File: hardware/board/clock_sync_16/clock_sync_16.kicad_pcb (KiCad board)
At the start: 4 copper layers, 36 x 28 mm, 47 parts, among them J2 AudioJack3, J3 USB_C_Receptacle_USB2.0, U1 TPD2EUSB30, U2 LP2985-3.3, U3 RP2040, U4 W25Q16JVUXIQ, X1 ECS-TXO-2016

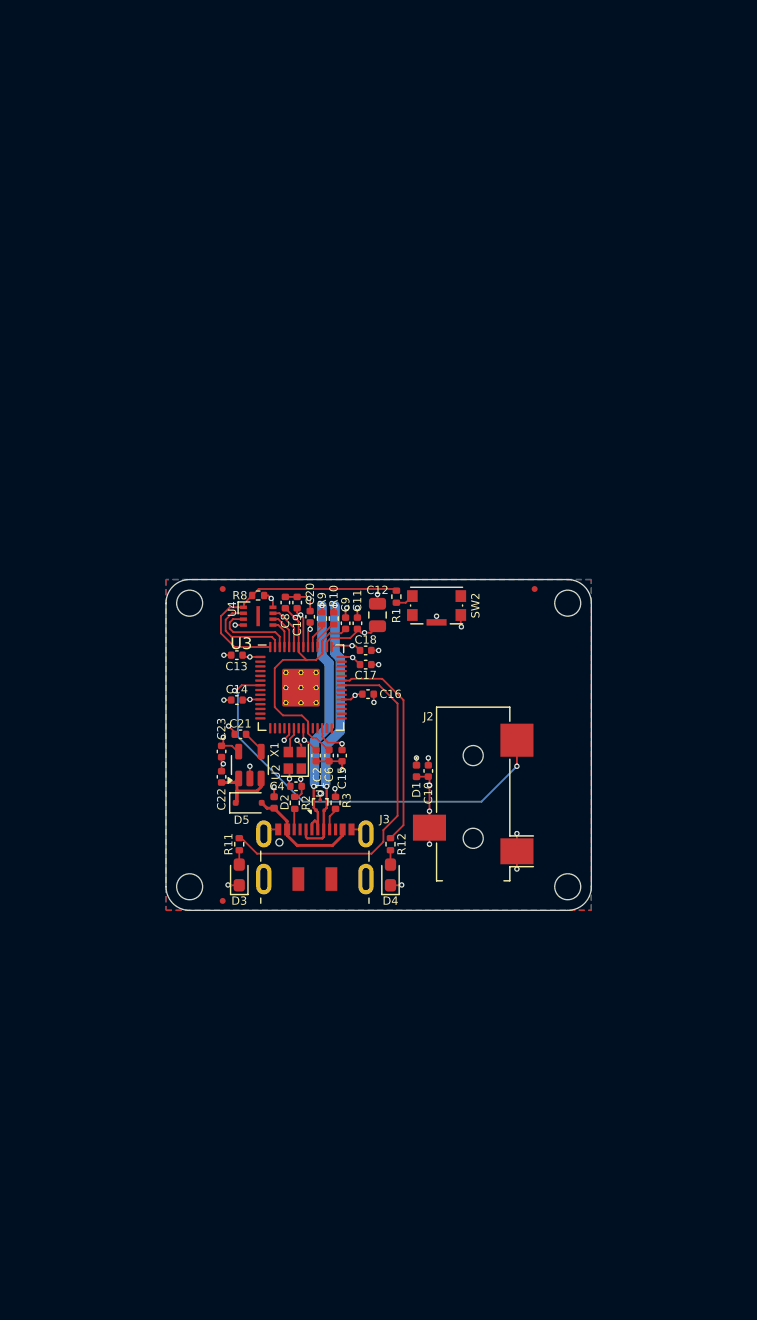
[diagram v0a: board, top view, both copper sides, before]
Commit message: route pcb v0.1
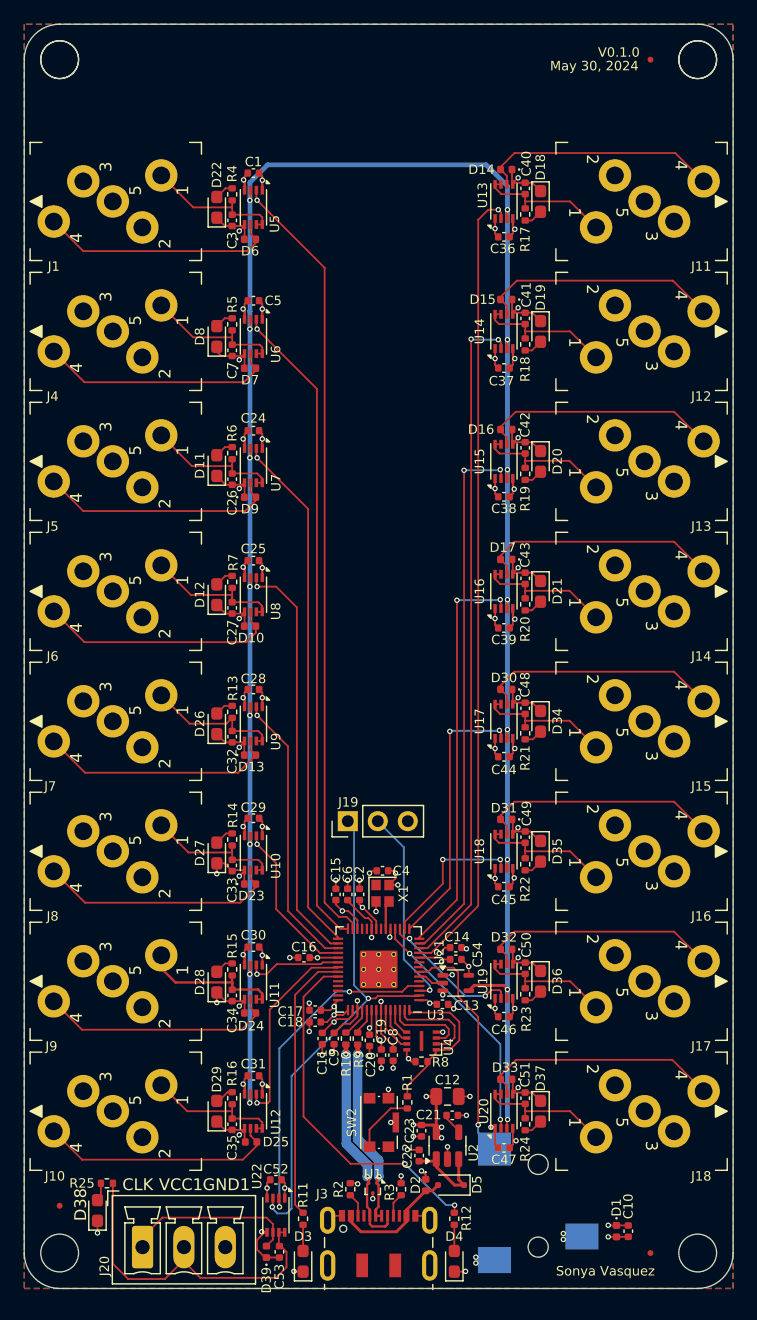
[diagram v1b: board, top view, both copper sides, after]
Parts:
- removed the REF** at (160.0, 84.0)
- removed the REF** at (128.0, 108.0)
- removed the REF** at (160.0, 108.0)
- removed the REF** at (128.0, 84.0)
- added ?: , , F.Cu at (117.0, 38.0)
- added ?: , , F.Cu at (171.0, 38.0)
- added C1: 1uF, Capacitor_SMD:C_0402_1005Metric, F.Cu at (133.4, 47.6)
- added C24: 1uF, Capacitor_SMD:C_0402_1005Metric, F.Cu at (133.4, 69.4)
- added C25: 1uF, Capacitor_SMD:C_0402_1005Metric, F.Cu at (133.4, 80.4)
- added C26: 1uF, Capacitor_SMD:C_0402_1005Metric, F.Cu at (131.6, 73.5)
- added C27: 1uF, Capacitor_SMD:C_0402_1005Metric, F.Cu at (131.6, 84.4)
- added C28: 1uF, Capacitor_SMD:C_0402_1005Metric, F.Cu at (133.4, 91.3)
- added C29: 1uF, Capacitor_SMD:C_0402_1005Metric, F.Cu at (133.4, 102.2)
- added C3: 1uF, Capacitor_SMD:C_0402_1005Metric, F.Cu at (131.6, 51.6)
- added C30: 1uF, Capacitor_SMD:C_0402_1005Metric, F.Cu at (133.4, 113.1)
- added C31: 1uF, Capacitor_SMD:C_0402_1005Metric, F.Cu at (133.4, 124.0)
- added C32: 1uF, Capacitor_SMD:C_0402_1005Metric, F.Cu at (131.6, 95.3)
- added C33: 1uF, Capacitor_SMD:C_0402_1005Metric, F.Cu at (131.6, 106.2)
- added C34: 1uF, Capacitor_SMD:C_0402_1005Metric, F.Cu at (131.6, 117.2)
- added C35: 1uF, Capacitor_SMD:C_0402_1005Metric, F.Cu at (131.6, 128.1)
- added C36: 1uF, Capacitor_SMD:C_0402_1005Metric, F.Cu at (154.6, 53.0)
- added C37: 1uF, Capacitor_SMD:C_0402_1005Metric, F.Cu at (154.6, 64.1)
- added C38: 1uF, Capacitor_SMD:C_0402_1005Metric, F.Cu at (154.6, 75.0)
- added C39: 1uF, Capacitor_SMD:C_0402_1005Metric, F.Cu at (154.6, 86.1)
- added C40: 1uF, Capacitor_SMD:C_0402_1005Metric, F.Cu at (156.4, 48.9)
- added C41: 1uF, Capacitor_SMD:C_0402_1005Metric, F.Cu at (156.4, 59.9)
- added C42: 1uF, Capacitor_SMD:C_0402_1005Metric, F.Cu at (156.4, 70.9)
- added C43: 1uF, Capacitor_SMD:C_0402_1005Metric, F.Cu at (156.4, 81.9)
- added C44: 1uF, Capacitor_SMD:C_0402_1005Metric, F.Cu at (154.6, 97.0)
- added C45: 1uF, Capacitor_SMD:C_0402_1005Metric, F.Cu at (154.6, 108.0)
- added C46: 1uF, Capacitor_SMD:C_0402_1005Metric, F.Cu at (154.6, 119.0)
- added C47: 1uF, Capacitor_SMD:C_0402_1005Metric, F.Cu at (154.6, 130.1)
- added C48: 1uF, Capacitor_SMD:C_0402_1005Metric, F.Cu at (156.4, 92.9)
- added C49: 1uF, Capacitor_SMD:C_0402_1005Metric, F.Cu at (156.4, 103.8)
- added C5: 1uF, Capacitor_SMD:C_0402_1005Metric, F.Cu at (133.4, 58.4)
- added C50: 1uF, Capacitor_SMD:C_0402_1005Metric, F.Cu at (156.4, 114.9)
- added C51: 1uF, Capacitor_SMD:C_0402_1005Metric, F.Cu at (156.4, 125.9)
- added C52: 1uF, Capacitor_SMD:C_0402_1005Metric, F.Cu at (135.3, 132.8)
- added C53: 1uF, Capacitor_SMD:C_0402_1005Metric, F.Cu at (135.6, 138.9)
- added C54: 1uF, Capacitor_SMD:C_0402_1005Metric, F.Cu at (150.5, 114.2)
- added C7: 1uF, Capacitor_SMD:C_0402_1005Metric, F.Cu at (131.6, 62.6)
- added D10: D_TVS, Diode_SMD:D_0402_1005Metric, F.Cu at (133.1, 85.9)
- added D11: LED, LED_SMD:LED_0603_1608Metric_Pad1.05x0.95mm_HandSolder, F.Cu at (130.3, 72.4)
- added D12: LED, LED_SMD:LED_0603_1608Metric_Pad1.05x0.95mm_HandSolder, F.Cu at (130.3, 83.3)
- added D13: D_TVS, Diode_SMD:D_0402_1005Metric, F.Cu at (133.1, 96.9)
- added D14: D_TVS, Diode_SMD:D_0402_1005Metric, F.Cu at (154.8, 47.3)
- added D15: D_TVS, Diode_SMD:D_0402_1005Metric, F.Cu at (154.8, 58.3)
- added D16: D_TVS, Diode_SMD:D_0402_1005Metric, F.Cu at (154.8, 69.3)
- added D17: D_TVS, Diode_SMD:D_0402_1005Metric, F.Cu at (154.8, 80.3)
- added D18: LED, LED_SMD:LED_0603_1608Metric_Pad1.05x0.95mm_HandSolder, F.Cu at (157.7, 50.0)
- added D19: LED, LED_SMD:LED_0603_1608Metric_Pad1.05x0.95mm_HandSolder, F.Cu at (157.7, 61.0)
- added D20: LED, LED_SMD:LED_0603_1608Metric_Pad1.05x0.95mm_HandSolder, F.Cu at (157.7, 72.0)
- added D21: LED, LED_SMD:LED_0603_1608Metric_Pad1.05x0.95mm_HandSolder, F.Cu at (157.7, 83.0)
- added D22: LED, LED_SMD:LED_0603_1608Metric_Pad1.05x0.95mm_HandSolder, F.Cu at (130.3, 50.5)
- added D23: D_TVS, Diode_SMD:D_0402_1005Metric, F.Cu at (133.1, 107.8)
- added D24: D_TVS, Diode_SMD:D_0402_1005Metric, F.Cu at (133.1, 118.7)
- added D25: D_TVS, Diode_SMD:D_0402_1005Metric, F.Cu at (133.2, 129.6)
- added D26: LED, LED_SMD:LED_0603_1608Metric_Pad1.05x0.95mm_HandSolder, F.Cu at (130.3, 94.2)
- added D27: LED, LED_SMD:LED_0603_1608Metric_Pad1.05x0.95mm_HandSolder, F.Cu at (130.3, 105.1)
- added D28: LED, LED_SMD:LED_0603_1608Metric_Pad1.05x0.95mm_HandSolder, F.Cu at (130.3, 116.1)
- added D29: LED, LED_SMD:LED_0603_1608Metric_Pad1.05x0.95mm_HandSolder, F.Cu at (130.3, 127.0)
- added D30: D_TVS, Diode_SMD:D_0402_1005Metric, F.Cu at (154.8, 91.3)
- added D31: D_TVS, Diode_SMD:D_0402_1005Metric, F.Cu at (154.8, 102.3)
- added D32: D_TVS, Diode_SMD:D_0402_1005Metric, F.Cu at (154.8, 113.3)
- added D33: D_TVS, Diode_SMD:D_0402_1005Metric, F.Cu at (154.8, 124.3)
- added D34: LED, LED_SMD:LED_0603_1608Metric_Pad1.05x0.95mm_HandSolder, F.Cu at (157.7, 94.0)
- added D35: LED, LED_SMD:LED_0603_1608Metric_Pad1.05x0.95mm_HandSolder, F.Cu at (157.7, 105.0)
- added D36: LED, LED_SMD:LED_0603_1608Metric_Pad1.05x0.95mm_HandSolder, F.Cu at (157.7, 116.0)
- added D37: LED, LED_SMD:LED_0603_1608Metric_Pad1.05x0.95mm_HandSolder, F.Cu at (157.7, 127.0)
- added D38: LED, LED_SMD:LED_0603_1608Metric_Pad1.05x0.95mm_HandSolder, F.Cu at (120.2, 135.4)
- added D39: D_TVS, Diode_SMD:D_0402_1005Metric, F.Cu at (134.5, 138.9)
- added D6: D_TVS, Diode_SMD:D_0402_1005Metric, F.Cu at (133.1, 53.2)
- added D7: D_TVS, Diode_SMD:D_0402_1005Metric, F.Cu at (133.1, 64.1)
- added D8: LED, LED_SMD:LED_0603_1608Metric_Pad1.05x0.95mm_HandSolder, F.Cu at (130.3, 61.4)
- added D9: D_TVS, Diode_SMD:D_0402_1005Metric, F.Cu at (133.1, 75.0)
- added J1: AudioJack3, kicad_component_library:Jack_3.5mm_Kycon_STX-3680-5NB_Vertical, F.Cu at (121.5, 50.0)
- added J10: AudioJack3, kicad_component_library:Jack_3.5mm_Kycon_STX-3680-5NB_Vertical, F.Cu at (121.5, 127.0)
- added J11: AudioJack3, kicad_component_library:Jack_3.5mm_Kycon_STX-3680-5NB_Vertical, F.Cu at (166.5, 50.0)
- added J12: AudioJack3, kicad_component_library:Jack_3.5mm_Kycon_STX-3680-5NB_Vertical, F.Cu at (166.5, 61.0)
- added J13: AudioJack3, kicad_component_library:Jack_3.5mm_Kycon_STX-3680-5NB_Vertical, F.Cu at (166.5, 72.0)
- added J14: AudioJack3, kicad_component_library:Jack_3.5mm_Kycon_STX-3680-5NB_Vertical, F.Cu at (166.5, 83.0)
- added J15: AudioJack3, kicad_component_library:Jack_3.5mm_Kycon_STX-3680-5NB_Vertical, F.Cu at (166.5, 94.0)
- added J16: AudioJack3, kicad_component_library:Jack_3.5mm_Kycon_STX-3680-5NB_Vertical, F.Cu at (166.5, 105.0)
- added J17: AudioJack3, kicad_component_library:Jack_3.5mm_Kycon_STX-3680-5NB_Vertical, F.Cu at (166.5, 116.0)
- added J18: AudioJack3, kicad_component_library:Jack_3.5mm_Kycon_STX-3680-5NB_Vertical, F.Cu at (166.5, 127.0)
- added J19: Conn_01x03_Male, Connector_PinHeader_2.54mm:PinHeader_1x03_P2.54mm_Vertical, F.Cu at (141.4, 102.5)
- added J20: Conn_01x03_Female, Connector_Phoenix_MC:PhoenixContact_MCV_1,5_3-G-3.5_1x03_P3.50mm_Vertical, F.Cu at (124.0, 138.5)
- added J4: AudioJack3, kicad_component_library:Jack_3.5mm_Kycon_STX-3680-5NB_Vertical, F.Cu at (121.5, 61.0)
- added J5: AudioJack3, kicad_component_library:Jack_3.5mm_Kycon_STX-3680-5NB_Vertical, F.Cu at (121.5, 72.0)
- added J6: AudioJack3, kicad_component_library:Jack_3.5mm_Kycon_STX-3680-5NB_Vertical, F.Cu at (121.5, 83.0)
- added J7: AudioJack3, kicad_component_library:Jack_3.5mm_Kycon_STX-3680-5NB_Vertical, F.Cu at (121.5, 94.0)
- added J8: AudioJack3, kicad_component_library:Jack_3.5mm_Kycon_STX-3680-5NB_Vertical, F.Cu at (121.5, 105.0)
- added J9: AudioJack3, kicad_component_library:Jack_3.5mm_Kycon_STX-3680-5NB_Vertical, F.Cu at (121.5, 116.0)
- added R13: R, Resistor_SMD:R_0402_1005Metric, F.Cu at (131.6, 93.2)
- added R14: R, Resistor_SMD:R_0402_1005Metric, F.Cu at (131.6, 104.0)
- added R15: R, Resistor_SMD:R_0402_1005Metric, F.Cu at (131.6, 115.0)
- added R16: R, Resistor_SMD:R_0402_1005Metric, F.Cu at (131.6, 125.9)
- added R17: R, Resistor_SMD:R_0402_1005Metric, F.Cu at (156.4, 51.1)
- added R18: R, Resistor_SMD:R_0402_1005Metric, F.Cu at (156.4, 62.1)
- added R19: R, Resistor_SMD:R_0402_1005Metric, F.Cu at (156.4, 73.1)
- added R20: R, Resistor_SMD:R_0402_1005Metric, F.Cu at (156.4, 84.1)
- added R21: R, Resistor_SMD:R_0402_1005Metric, F.Cu at (156.4, 95.0)
- added R22: R, Resistor_SMD:R_0402_1005Metric, F.Cu at (156.4, 106.1)
- added R23: R, Resistor_SMD:R_0402_1005Metric, F.Cu at (156.4, 117.1)
- added R24: R, Resistor_SMD:R_0402_1005Metric, F.Cu at (156.4, 128.1)
- added R25: R, Resistor_SMD:R_0402_1005Metric, F.Cu at (121.0, 133.1)
- added R4: R, Resistor_SMD:R_0402_1005Metric, F.Cu at (131.6, 49.4)
- added R5: R, Resistor_SMD:R_0402_1005Metric, F.Cu at (131.6, 60.4)
- added R6: R, Resistor_SMD:R_0402_1005Metric, F.Cu at (131.6, 71.3)
- added R7: R, Resistor_SMD:R_0402_1005Metric, F.Cu at (131.6, 82.2)
- added REF**: MountingHole_3.2mm_M3_DIN965, MountingHole:MountingHole_3.2mm_M3_DIN965, F.Cu at (117.0, 38.0)
- added REF**: MountingHole_3.2mm_M3_DIN965, MountingHole:MountingHole_3.2mm_M3_DIN965, F.Cu at (117.0, 139.0)
- added REF**: MountingHole_3.2mm_M3_DIN965, MountingHole:MountingHole_3.2mm_M3_DIN965, F.Cu at (171.0, 38.0)
- added REF**: MountingHole_3.2mm_M3_DIN965, MountingHole:MountingHole_3.2mm_M3_DIN965, F.Cu at (171.0, 139.0)
- added U10: ISO6521FREUR, kicad_component_library:DFN-8_3x2mm_P0.5mm, F.Cu at (133.4, 105.1)
- added U11: ISO6521FREUR, kicad_component_library:DFN-8_3x2mm_P0.5mm, F.Cu at (133.4, 116.1)
- added U12: ISO6521FREUR, kicad_component_library:DFN-8_3x2mm_P0.5mm, F.Cu at (133.4, 127.0)
- added U13: ISO6521FREUR, kicad_component_library:DFN-8_3x2mm_P0.5mm, F.Cu at (154.6, 50.0)
- added U14: ISO6521FREUR, kicad_component_library:DFN-8_3x2mm_P0.5mm, F.Cu at (154.6, 61.0)
- added U15: ISO6521FREUR, kicad_component_library:DFN-8_3x2mm_P0.5mm, F.Cu at (154.6, 72.0)
- added U16: ISO6521FREUR, kicad_component_library:DFN-8_3x2mm_P0.5mm, F.Cu at (154.6, 83.0)
- added U17: ISO6521FREUR, kicad_component_library:DFN-8_3x2mm_P0.5mm, F.Cu at (154.6, 94.0)
- added U18: ISO6521FREUR, kicad_component_library:DFN-8_3x2mm_P0.5mm, F.Cu at (154.6, 105.0)
- added U19: ISO6521FREUR, kicad_component_library:DFN-8_3x2mm_P0.5mm, F.Cu at (154.6, 116.0)
- added U20: ISO6521FREUR, kicad_component_library:DFN-8_3x2mm_P0.5mm, F.Cu at (154.6, 127.0)
- added U21: SN74LVC1G125DCK, Package_TO_SOT_SMD:Texas_R-PDSO-G5_DCK-5, F.Cu at (150.5, 116.2)
- added U22: ISO6521FREUR, kicad_component_library:DFN-8_3x2mm_P0.5mm, F.Cu at (135.3, 135.8)
- added U5: ISO6521FREUR, kicad_component_library:DFN-8_3x2mm_P0.5mm, F.Cu at (133.4, 50.5)
- added U6: ISO6521FREUR, kicad_component_library:DFN-8_3x2mm_P0.5mm, F.Cu at (133.4, 61.4)
- added U7: ISO6521FREUR, kicad_component_library:DFN-8_3x2mm_P0.5mm, F.Cu at (133.4, 72.4)
- added U8: ISO6521FREUR, kicad_component_library:DFN-8_3x2mm_P0.5mm, F.Cu at (133.4, 83.3)
- added U9: ISO6521FREUR, kicad_component_library:DFN-8_3x2mm_P0.5mm, F.Cu at (133.4, 94.2)
- J2: moved to B.Cu
- moved FID3 79.9 mm to (167.0, 38.0)
- moved FID2 57.0 mm to (167.0, 139.0)
- moved FID1 54.0 mm to (117.0, 135.0)
- moved SW2 44.0 mm to (144.0, 128.0), turned to -90 degrees
- moved R1 42.8 mm to (146.4, 126.2)
- moved C10 42.5 mm to (165.1, 137.2)
- moved D1 42.5 mm to (164.1, 137.2)
- moved R8 41.8 mm to (147.6, 122.8), turned to 180 degrees
- moved C12 41.2 mm to (149.8, 125.8), turned to 0 degrees
- moved C8 39.4 mm to (145.2, 122.2), turned to 90 degrees
- moved C19 39.0 mm to (144.2, 122.2), turned to 90 degrees
- moved U4 38.5 mm to (147.6, 121.0), turned to 180 degrees
- moved C21 36.9 mm to (150.2, 127.3), turned to 0 degrees
- moved D5 36.6 mm to (150.1, 133.2), turned to 180 degrees
- moved U2 36.3 mm to (149.8, 129.9)
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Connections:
- net +3V3 renamed +3.3V
- net /Harp Core RP2040 + USB/HARP_CLK_SYNC renamed /Harp Core RP2040 + USB/HARP_CLKIN_SYNC
- U3 pad 11: unconnected-(U3-GPIO8-Pad11) -> /Clock Outputs 8 - 16/CH8_CONNECTED
- U3 pad 12: unconnected-(U3-GPIO9-Pad12) -> /Clock Outputs 8 - 16/CH9_CONNECTED
- U3 pad 13: unconnected-(U3-GPIO10-Pad13) -> /Clock Outputs 8 - 16/CH10_CONNECTED
- U3 pad 14: unconnected-(U3-GPIO11-Pad14) -> /Clock Outputs 8 - 16/CH11_CONNECTED
- U3 pad 15: unconnected-(U3-GPIO12-Pad15) -> /Clock Outputs 8 - 16/CH12_CONNECTED
- U3 pad 16: unconnected-(U3-GPIO13-Pad16) -> /Clock Outputs 8 - 16/CH13_CONNECTED
- U3 pad 17: unconnected-(U3-GPIO14-Pad17) -> /Clock Outputs 8 - 16/CH14_CONNECTED
- U3 pad 18: unconnected-(U3-GPIO15-Pad18) -> /Clock Outputs 8 - 16/CH15_CONNECTED
- U3 pad 2: unconnected-(U3-GPIO0-Pad2) -> /Harp Core RP2040 + USB/SLOW_CLKOUT
- U3 pad 27: unconnected-(U3-GPIO16-Pad27) -> /Clock Outputs 0 - 7/CH0_CONNECTED
- U3 pad 28: unconnected-(U3-GPIO17-Pad28) -> /Clock Outputs 0 - 7/CH1_CONNECTED
- U3 pad 29: unconnected-(U3-GPIO18-Pad29) -> /Clock Outputs 0 - 7/CH2_CONNECTED
- U3 pad 3: unconnected-(U3-GPIO1-Pad3) -> /Harp Core RP2040 + USB/UART0_RXD
- U3 pad 30: unconnected-(U3-GPIO19-Pad30) -> /Clock Outputs 0 - 7/CH3_CONNECTED
- U3 pad 31: unconnected-(U3-GPIO20-Pad31) -> /Clock Outputs 0 - 7/CH4_CONNECTED
- U3 pad 32: unconnected-(U3-GPIO21-Pad32) -> /Clock Outputs 0 - 7/CH5_CONNECTED
- U3 pad 34: unconnected-(U3-GPIO22-Pad34) -> /Clock Outputs 0 - 7/CH6_CONNECTED
- U3 pad 35: unconnected-(U3-GPIO23-Pad35) -> /Clock Outputs 0 - 7/CH7_CONNECTED
- U3 pad 4: unconnected-(U3-GPIO2-Pad4) -> /Harp Core RP2040 + USB/SLOW_CLKOUT_CONNECTED
- U3 pad 6: unconnected-(U3-GPIO4-Pad6) -> /Harp Core RP2040 + USB/HARP_CLKOUT
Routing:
- net HARP_CLKOUT: track 0.00 -> 196.3 mm, vias 0 -> 16
- net /Clock Outputs 8 - 16/CH8_CONNECTED: track 0.00 -> 67.6 mm, vias 0 -> 1
- net /Clock Outputs 0 - 7/CH0_CONNECTED: track 0.00 -> 66.3 mm, vias 0 -> 1
- net /Clock Outputs 8 - 16/CH9_CONNECTED: track 0.00 -> 56.9 mm, vias 0 -> 2
- net /Clock Outputs 0 - 7/CH1_CONNECTED: track 0.00 -> 55.6 mm, vias 0 -> 1
- net /Clock Outputs 8 - 16/CH10_CONNECTED: track 0.00 -> 45.7 mm, vias 0 -> 2
- net /Clock Outputs 0 - 7/CH2_CONNECTED: track 0.00 -> 44.4 mm, vias 0 -> 1
- net /Harp Core RP2040 + USB/SLOW_CLKOUT: track 0.00 -> 43.6 mm, vias 0 -> 2
- net +3.3V: track 38.6 -> 80.2 mm, vias 16 -> 38
- net GND: track 32.4 -> 72.4 mm, vias 28 -> 53
- net /Clock Outputs 0 - 7/CH3_CONNECTED: track 0.00 -> 35.1 mm, vias 0 -> 1
- net /Clock Outputs 8 - 16/CH11_CONNECTED: track 0.00 -> 34.4 mm, vias 0 -> 2
- net Net-(J20-Pin_2): track 0.00 -> 29.7 mm
- net /Harp Core RP2040 + USB/SLOW_CLKOUT_CONNECTED: track 0.00 -> 28.3 mm, vias 0 -> 2
- net /Clock Outputs 0 - 7/CH4_CONNECTED: track 0.00 -> 23.9 mm, vias 0 -> 1
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- added copper zone on In2.Cu, net +1V1
- added copper zone on In1.Cu, net Net-(D10-A1)
- added copper zone on In1.Cu, net Net-(D11-K)
- added copper zone on In1.Cu, net Net-(D13-A1)
- added copper zone on In1.Cu, net Net-(D14-A1)
- added copper zone on In1.Cu, net Net-(D15-A1)
- added copper zone on In1.Cu, net Net-(D16-A1)
- added copper zone on In1.Cu, net Net-(D17-A1)
- added copper zone on In1.Cu, net Net-(D22-K)
- added copper zone on In1.Cu, net Net-(D23-A1)
- added copper zone on In1.Cu, net Net-(D24-A1)
- added copper zone on In1.Cu, net Net-(D25-A1)
- added copper zone on In1.Cu, net Net-(D30-A1)
- added copper zone on In1.Cu, net Net-(D31-A1)
- added copper zone on In1.Cu, net Net-(D32-A1)
- added copper zone on In1.Cu, net Net-(D33-A1)
- added copper zone on In1.Cu, net Net-(D38-K)
- added copper zone on In1.Cu, net Net-(D7-A1)
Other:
- board size 36 x 28 mm -> 60 x 107 mm
- board text added: "CLK"
- board text added: "GND1"
- board text added: "May 30, 2024"
- board text added: "Sonya Vasquez"
- board text added: "V0.1.0"
- board text added: "VCC1"
- board text removed: "1"
- board text removed: "V0.1.1"
